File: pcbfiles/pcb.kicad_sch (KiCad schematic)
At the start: 236 parts, among them J1 Conn_01x06, J2 Conn_01x06, J3 Conn_01x06, J4 Conn_01x06, J5 Conn_01x04_Female, J6 Conn_01x04_Female, Q1 AO3401A, Q2 AO3401A, SW1 SW_SPST, SW10 SW_SPST, SW11 SW_SPST, SW12 SW_SPST, SW13 SW_SPST, SW14 SW_SPST, SW15 SW_SPST, SW16 SW_SPST, SW17 SW_SPST, SW18 SW_SPST, SW19 SW_SPST, SW2 SW_SPST, SW20 SW_SPST, SW21 SW_SPST, SW22 SW_SPST, SW23 SW_SPST, SW24 SW_SPST, SW25 SW_SPST, SW26 SW_SPST, SW27 SW_SPST, SW28 SW_SPST, SW29 SW_SPST, SW3 SW_SPST, SW30 SW_SPST, SW31 SW_SPST, SW32 SW_SPST, SW33 SW_SPST, SW34 SW_SPST, SW35 SW_SPST, SW36 SW_SPST, SW37 SW_SPST, SW38 SW_SPST, SW39 SW_SPST, SW4 SW_SPST, SW40 SW_SPST, SW41 SW_SPST, SW42 SW_SPST, SW43 SW_SPST, SW44 SW_SPST, SW45 SW_SPST, SW46 SW_SPST, SW47 SW_SPST, SW48 SW_SPST, SW49 SW_SPST, SW5 SW_SPST, SW50 SW_SPST, SW51 SW_SPST, SW52 SW_SPST, SW53 SW_SPST, SW54 SW_SPST, SW55 SW_SPST, SW56 SW_SPST, SW57 SW_SPST, SW58 SW_SPST, SW59 SW_SPST, SW6 SW_SPST, SW60 SW_SPST, SW61 SW_SPST, SW62 SW_SPST, SW63 SW_SPST, SW64 SW_SPST, SW65 SW_SPST, SW66 SW_SPST, SW67 SW_SPST, SW68 SW_SPST, SW69 SW_SPST, SW7 SW_SPST, SW70 SW_SPST, SW71 SW_SPST, SW72 SW_SPST, SW73 SW_SPST, SW74 SW_SPST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

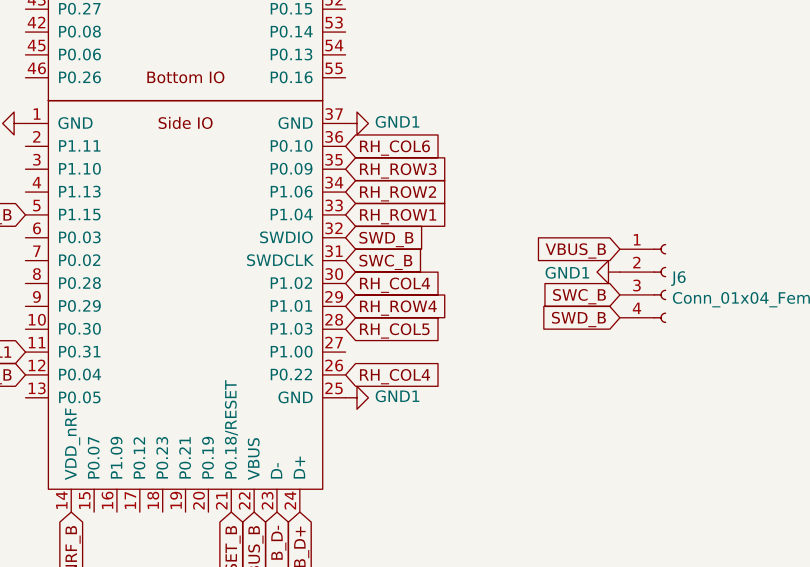
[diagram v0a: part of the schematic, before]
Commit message: Routing.
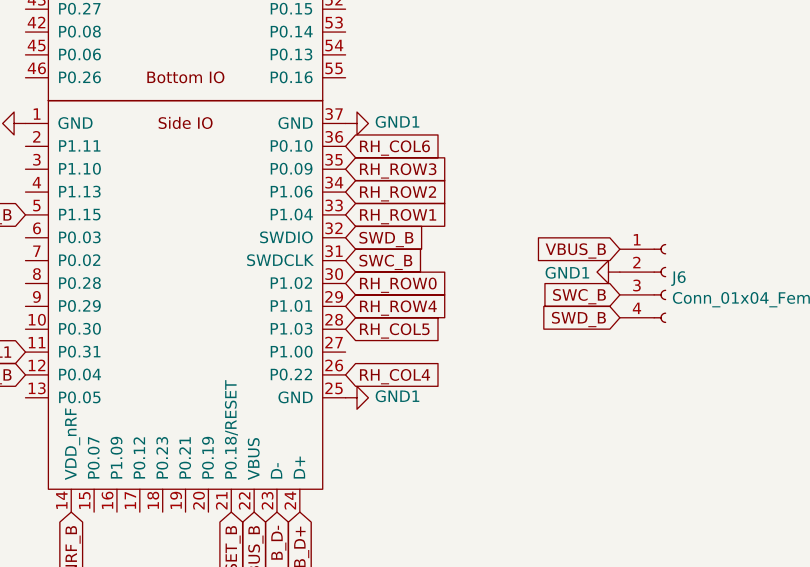
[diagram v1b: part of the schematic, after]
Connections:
- net RH_COL4: no longer U6.30 (P1.02)
- net RH_ROW0: now also U6.30 (P1.02)
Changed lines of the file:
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@@
     )
   )
-  (global_label "RH_COL4" (shape input) (at 525.272 262.89 0) (fields_autoplaced)
+  (global_label "RH_ROW0" (shape input) (at 525.272 262.89 0) (fields_autoplaced)
     (effects (font (size 1.27 1.27)) (justify left))
-    (property "Intersheet References" "${INTERSHEET_REFS}" (id 0) (at 609.092 -346.71 0)
-      (effects (font (size 1.27 1.27)) hide)
+    (property "Intersheet References" "${INTERSHEET_REFS}" (id 0) (at 536.4257 262.8106 0)
+      (effects (font (size 1.27 1.27)) (justify left) hide)
     )
   )

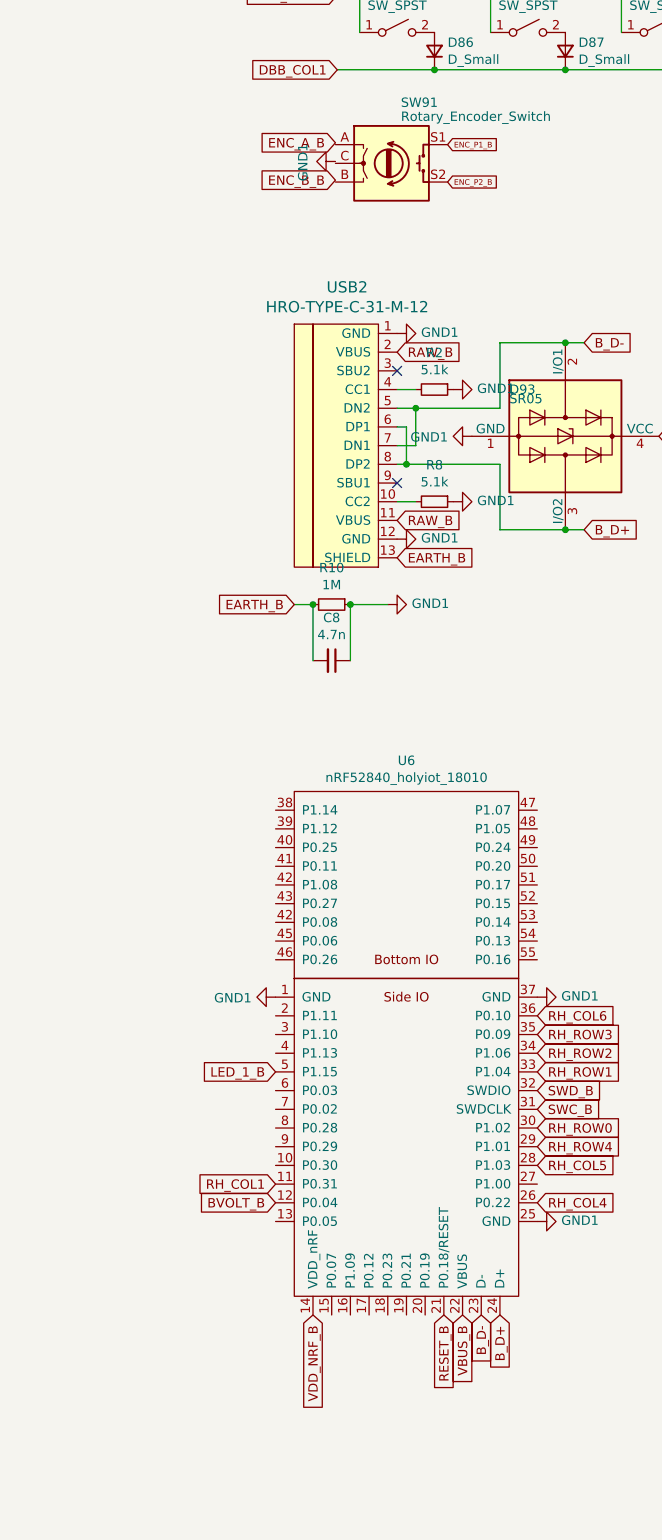
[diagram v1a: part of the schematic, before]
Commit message: Routing.
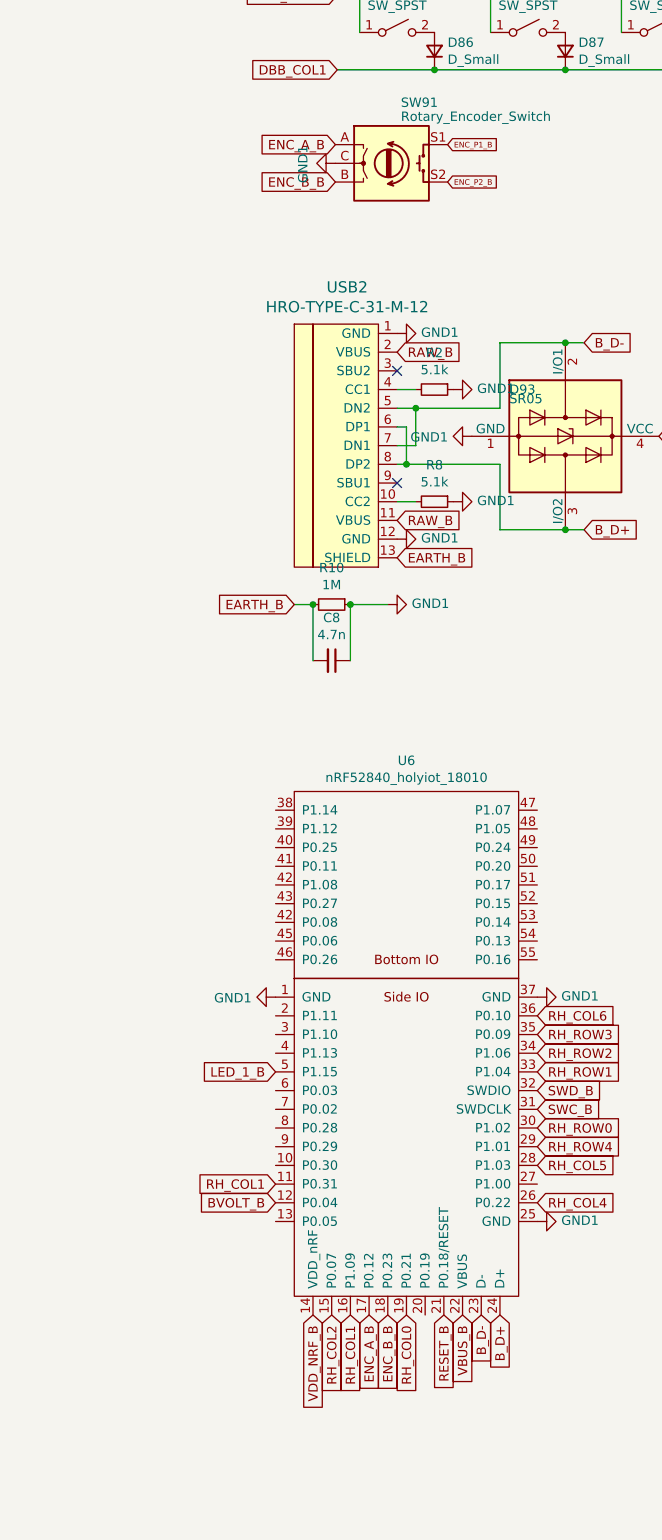
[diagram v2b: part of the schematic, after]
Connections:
- net ENC_A_B: now also SW91.A, U6.17 (P0.12)
- net ENC_B_B: now also SW91.B, U6.18 (P0.23)
- net ENC_P1_B: now also U6.19 (P0.21)
- net GND1: now also SW91.C
- net RH_COL1: now also U6.16 (P1.09)
- net RH_COL2: now also U6.15 (P0.07)
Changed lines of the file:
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@@
+    )
+  )
+  (global_label "ENC_B_B" (shape input) (at 504.952 288.29 270) (fields_autoplaced)
+    (effects (font (size 1.27 1.27)) (justify right))
+    (property "Intersheet References" "${INTERSHEET_REFS}" (id 0) (at 505.0314 298.839 90)
+      (effects (font (size 1.27 1.27)) (justify right) hide)
     )
   )
@@
     )
   )
-  (global_label "ENC_A_B" (shape input) (at 497.84 129.032 180) (fields_autoplaced)
-    (effects (font (size 1.27 1.27)) (justify right))
-    (property "Intersheet References" "${INTERSHEET_REFS}" (id 0) (at 487.4725 129.1114 0)
+  (global_label "ENC_A_B" (shape input) (at 497.84 129.286 180) (fields_autoplaced)
+    (effects (font (size 1.27 1.27)) (justify right))
+    (property "Intersheet References" "${INTERSHEET_REFS}" (id 0) (at 487.4725 129.3654 0)
       (effects (font (size 1.27 1.27)) (justify right) hide)
     )
@@
     )
   )
+  (global_label "RH_COL2" (shape input) (at 497.332 288.29 270) (fields_autoplaced)
+    (effects (font (size 1.27 1.27)) (justify right))
+    (property "Intersheet References" "${INTERSHEET_REFS}" (id 0) (at 497.2526 299.0204 90)
+      (effects (font (size 1.27 1.27)) (justify right) hide)
+    )
+  )
   (global_label "VBAT_B" (shape input) (at 567.182 199.39 180) (fields_autoplaced)
     (effects (font (size 1.27 1.27)) (justify right))
@@
     )
   )
-  (global_label "ENC_B_B" (shape input) (at 497.84 134.112 180) (fields_autoplaced)
-    (effects (font (size 1.27 1.27)) (justify right))
-    (property "Intersheet References" "${INTERSHEET_REFS}" (id 0) (at 487.291 134.1914 0)
+  (global_label "ENC_B_B" (shape input) (at 497.84 134.366 180) (fields_autoplaced)
+    (effects (font (size 1.27 1.27)) (justify right))
+    (property "Intersheet References" "${INTERSHEET_REFS}" (id 0) (at 487.291 134.4454 0)
       (effects (font (size 1.27 1.27)) (justify right) hide)
     )
@@
     (property "Intersheet References" "${INTERSHEET_REFS}" (id 0) (at -100.33 -72.39 0)
       (effects (font (size 1.27 1.27)) hide)
+    )
+  )
+  (global_label "ENC_A_B" (shape input) (at 502.412 288.29 270) (fields_autoplaced)
+    (effects (font (size 1.27 1.27)) (justify right))
+    (property "Intersheet References" "${INTERSHEET_REFS}" (id 0) (at 502.4914 298.6575 90)
+      (effects (font (size 1.27 1.27)) (justify right) hide)
     )
   )
@@
     )
   )
+  (global_label "RH_COL1" (shape input) (at 499.872 288.29 270) (fields_autoplaced)
+    (effects (font (size 1.27 1.27)) (justify right))
+    (property "Intersheet References" "${INTERSHEET_REFS}" (id 0) (at 499.7926 299.0204 90)
+      (effects (font (size 1.27 1.27)) (justify right) hide)
+    )
+  )
   (global_label "DBA_P5" (shape input) (at 164.592 105.918 180) (fields_autoplaced)
     (effects (font (size 1.27 1.27)) (justify right))
@@
     (effects (font (size 1.27 1.27)) (justify left))
     (property "Intersheet References" "${INTERSHEET_REFS}" (id 0) (at 609.092 -397.51 0)
+      (effects (font (size 1.27 1.27)) hide)
+    )
+  )
+  (global_label "RH_COL0" (shape input) (at 507.492 288.29 270) (fields_autoplaced)
+    (effects (font (size 1.27 1.27)) (justify right))
+    (property "Intersheet References" "${INTERSHEET_REFS}" (id 0) (at 1045.972 372.11 0)
       (effects (font (size 1.27 1.27)) hide)
     )
@@
     (pin "1")
   )
-  (symbol (lib_id "power:GND1") (at 497.84 131.572 270) (unit 1)
-    (in_bom yes) (on_board yes)
-    (property "Reference" "#PWR02" (id 0) (at 491.49 131.572 0)
-      (effects (font (size 1.27 1.27)) hide)
-    )
-    (property "Value" "GND1" (id 1) (at 493.4458 131.699 0))
-    (property "Footprint" "" (id 2) (at 497.84 131.572 0)
-      (effects (font (size 1.27 1.27)) hide)
-    )
-    (property "Datasheet" "" (id 3) (at 497.84 131.572 0)
-      (effects (font (size 1.27 1.27)) hide)
-    )
+  (symbol (lib_id "power:GND1") (at 497.84 131.826 270) (unit 1)
+    (in_bom yes) (on_board yes)
+    (property "Reference" "#PWR02" (id 0) (at 491.49 131.826 0)
+      (effects (font (size 1.27 1.27)) hide)
+    )
+    (property "Value" "GND1" (id 1) (at 493.4458 131.953 0))
+    (property "Footprint" "" (id 2) (at 497.84 131.826 0)
+      (effects (font (size 1.27 1.27)) hide)
+    )
+    (property "Datasheet" "" (id 3) (at 497.84 131.826 0)
+      (effects (font (size 1.27 1.27)) hide)
+    )
